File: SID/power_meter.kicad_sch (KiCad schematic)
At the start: 0 parts

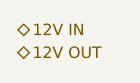
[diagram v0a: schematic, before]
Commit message: Feat(SID): basically complete
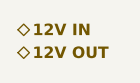
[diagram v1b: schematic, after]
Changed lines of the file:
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@@
-(kicad_sch (version 20230819) (generator eeschema)
-  (paper "A4")
-  (hierarchical_label "12V IN" (shape bidirectional) (at 88.9 97.79 0) (fields_autoplaced)
-    (effects (font (size 1.27 1.27)) (justify left))
-  )
-  (hierarchical_label "12V OUT" (shape bidirectional) (at 88.9 100.33 0) (fields_autoplaced)
-    (effects (font (size 1.27 1.27)) (justify left))
-  )
+(kicad_sch
+	(version 20240101)
+	(generator "eeschema")
+	(generator_version "8.99")
+	(paper "A4")
+	(hierarchical_label "12V IN"
+		(shape bidirectional)
+		(at 88.9 97.79 0)
+		(fields_autoplaced yes)
+		(effects
+			(font
+				(face "JetBrains Mono")
+				(size 1.27 1.27)
+				(thickness 0.254)
+				(bold yes)
+			)
+			(justify left)
+		)
+	)
+	(hierarchical_label "12V OUT"
+		(shape bidirectional)
+		(at 88.9 100.33 0)
+		(fields_autoplaced yes)
+		(effects
+			(font
+				(face "JetBrains Mono")
+				(size 1.27 1.27)
+				(thickness 0.254)
+				(bold yes)
+			)
+			(justify left)
+		)
+	)
 )
